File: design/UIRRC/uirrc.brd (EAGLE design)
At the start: 47.9 x 80.6 mm, 29 parts, among them IC1 TSOP38438, IC2 MIC5205-3.3YM5-TR, SW1 OMRON_B3SN-3112POMRON_B3SN-31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, SW2 OMRON_B3SN-3112POMRON_B3SN-31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, SW3 OMRON_B3SN-3112POMRON_B3SN-31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, SW4 OMRON_B3SN-3112POMRON_B3SN-31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, SW5 OMRON_B3SN-3112POMRON_B3SN-31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, SW6 OMRON_B3SN-3112POMRON_B3SN-31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, SW7 OMRON_B3SN-3112POMRON_B3SN-31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, SW8 OMRON_B3SN-3112POMRON_B3SN-31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, SW9 OMRON_B3SN-3112POMRON_B3SN-31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, U1 2479, U2 ESP32-WROOM-32E_(16MB)

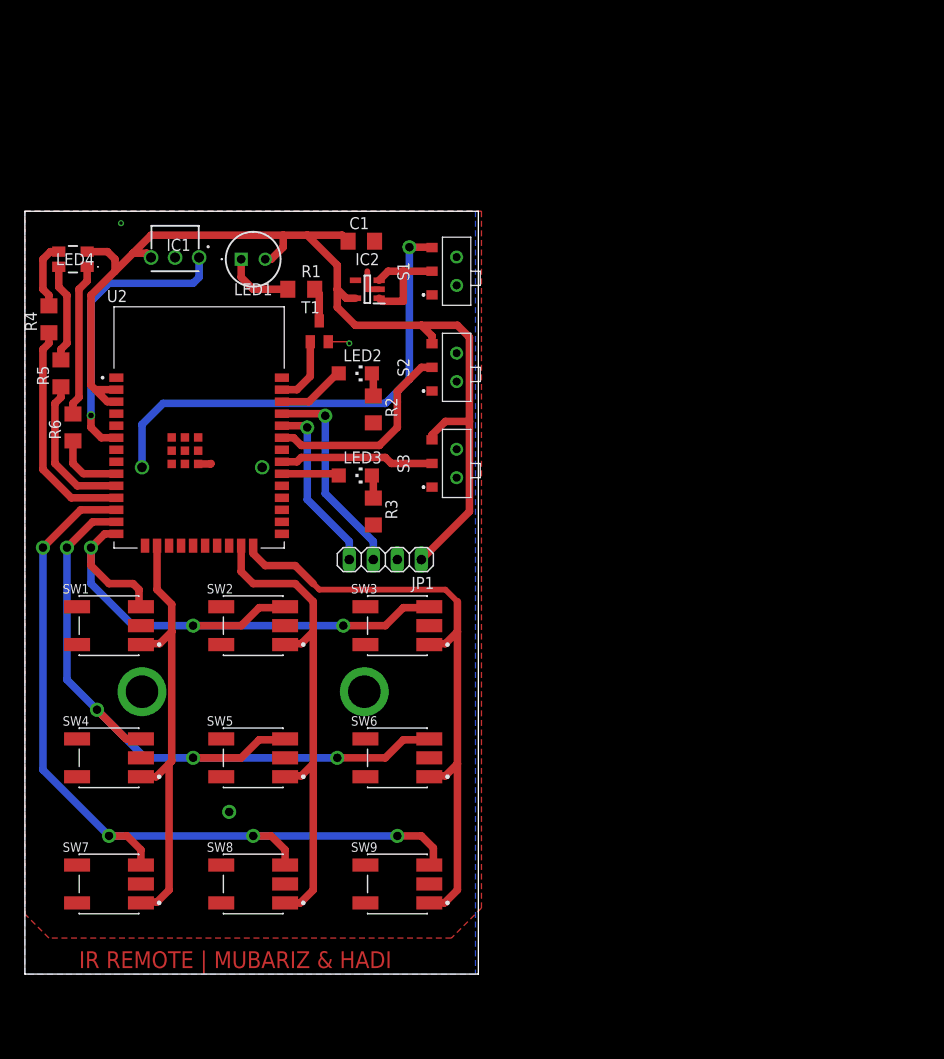
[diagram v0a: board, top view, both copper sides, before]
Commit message: add uml
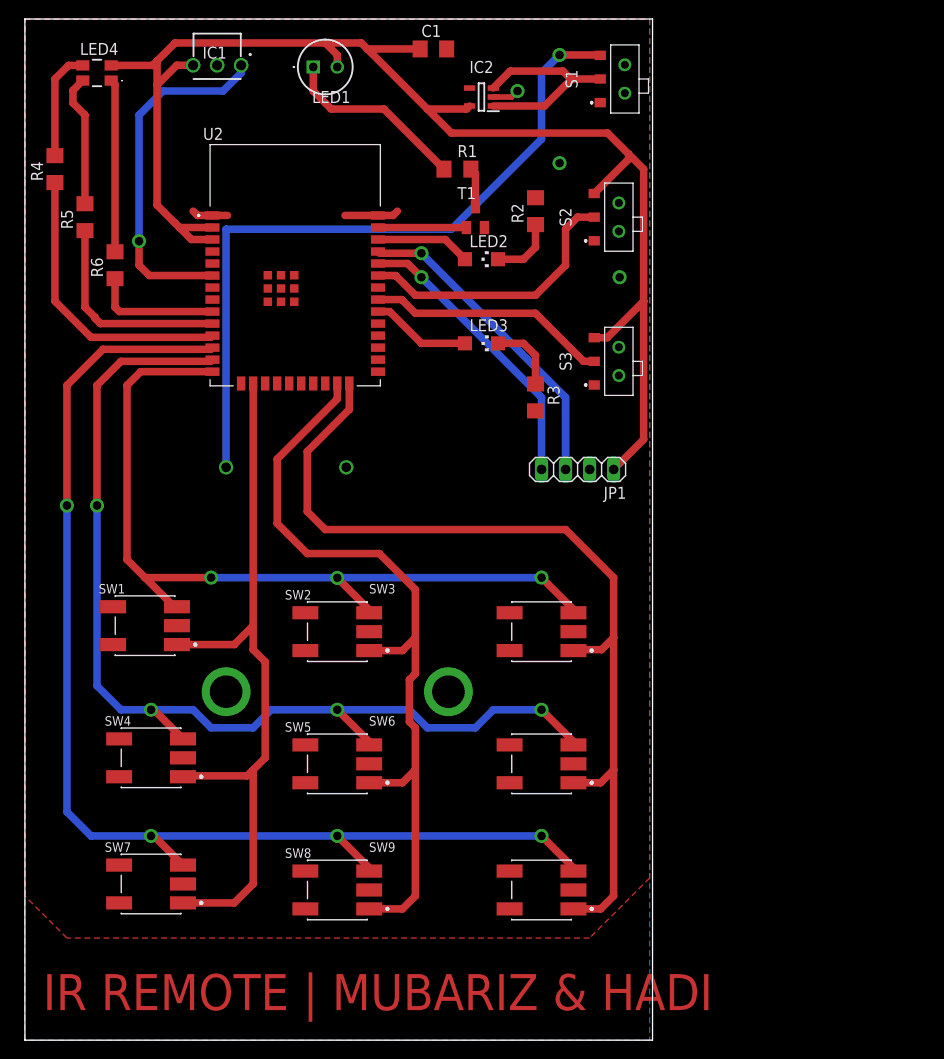
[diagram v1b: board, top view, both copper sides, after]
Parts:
- moved R2 27.1 mm to (54.0, 80.6), turned to 90 degrees
- moved S1 27.0 mm to (62.9, 94.6)
- moved IC2 23.6 mm to (48.3, 92.7)
- moved S2 23.4 mm to (62.2, 80.0)
- moved JP1 22.4 mm to (58.4, 53.3)
- moved C1 21.7 mm to (43.2, 97.8)
- moved LED1 21.7 mm to (30.5, 95.9)
- moved R3 21.0 mm to (54.0, 61.0)
- moved R1 20.8 mm to (45.7, 85.1)
- moved IC1 20.8 mm to (20.3, 94.6)
- moved T1 20.4 mm to (47.6, 80.0)
- moved S3 20.3 mm to (62.2, 64.8)
- moved U2 19.9 mm to (28.6, 74.9)
- moved LED4 19.8 mm to (7.62, 95.2)
- moved LED3 19.3 mm to (48.3, 66.7)
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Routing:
- net BUTTON_R3: track 91.0 -> 128.2 mm
- net +3V3: track 117.6 -> 152.4 mm
- net BUTTON_C3: track 65.6 -> 98.7 mm
- net BUTTON_R2: track 79.3 -> 111.2 mm
- net BUTTON_C2: track 52.8 -> 84.2 mm
- net BUTTON_C1: track 48.2 -> 78.8 mm
- net N$11: track 51.1 -> 76.5 mm
- net BUTTON_R1: track 66.0 -> 87.5 mm
- net N$1: track 7.36 -> 19.8 mm
- net USB_TXD: track 18.6 -> 30.8 mm
- net USB_RXD: track 22.0 -> 33.8 mm
- net N$16: track 11.9 -> 21.8 mm
- net LEARN_EN: track 16.3 -> 25.6 mm
- net WIFI_EN: track 21.9 -> 29.4 mm
- net N$13: track 23.7 -> 30.9 mm
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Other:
- board size 47.9 x 80.6 mm -> 66.3 x 107.9 mm
